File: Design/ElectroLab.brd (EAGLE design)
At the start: 175 x 100 mm, 232 parts, among them IC1 LM2902DT, IC10 CD4511BNSR, IC11 PAM8403, IC13 ADXL337, IC14 MIC5205, IC2 LM2902DT, IC3 SN74LV08ADR, IC4 SN74LV32ADR, IC5 SN74LV04ADR, IC6 4027D, IC7 4027D, IC8 NE555D, U1 USB, U2 GAS_SENSOR

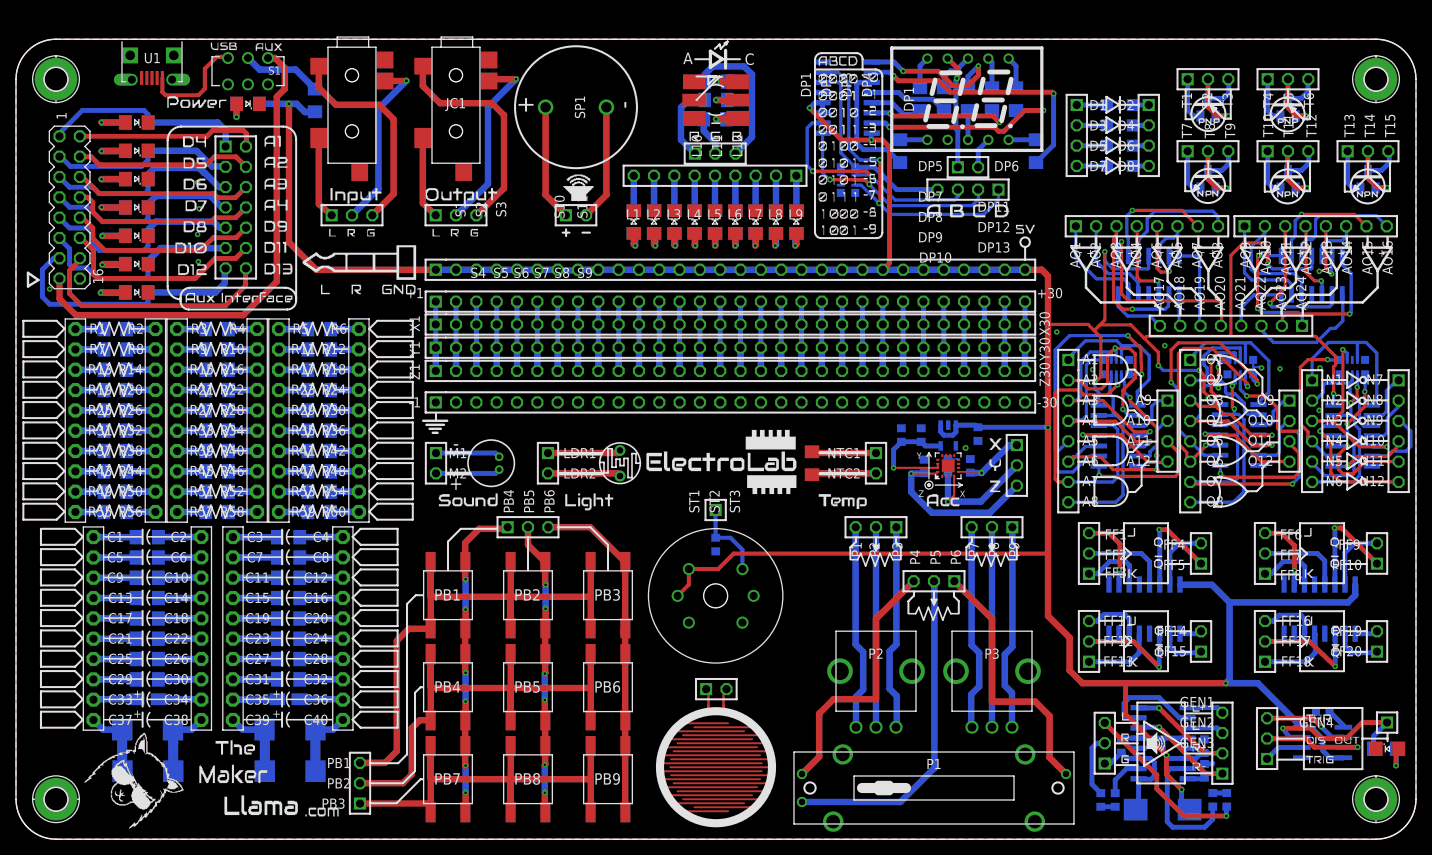
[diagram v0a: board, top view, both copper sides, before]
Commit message: Updated V3R1
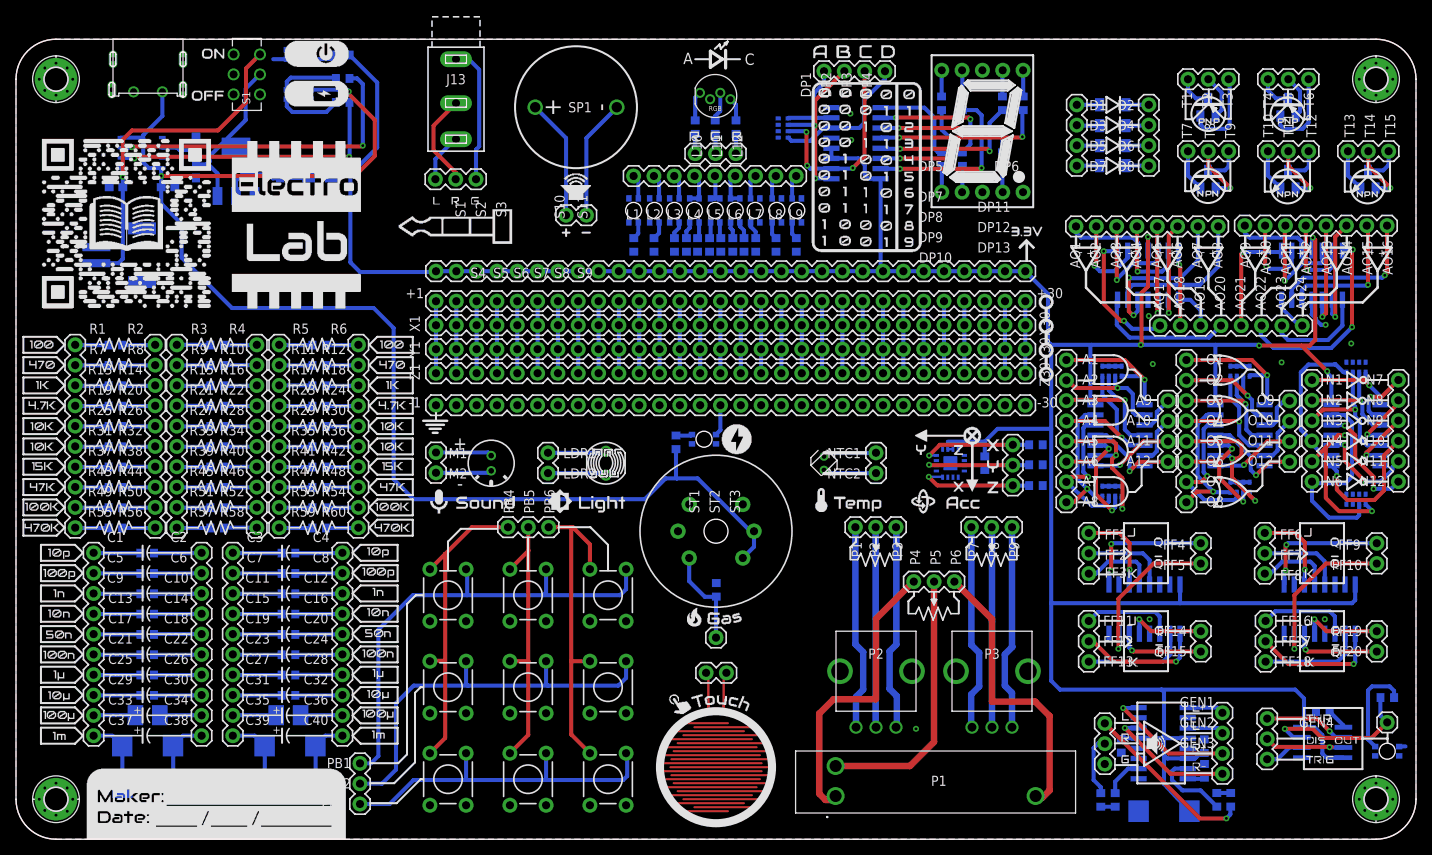
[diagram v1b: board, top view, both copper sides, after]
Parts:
- removed AR1, AR2, AR3, AR4: 1K, SpaceDIY:RESISTOR_ARRAY_X8_CAY17
- removed C33, C34: 10uF, SpaceDIY_passive_components:0603
- removed D1, D2, D3, D4: (no value), Seeed-OPL-Diode:LED-1206
- removed DP1: 2X7_SEGMENT_COMMON_CATODE_12_PINS, SpaceDIY:2X7_SEGMENT_COMMON_CATODE_12_PINS
- removed IC1, IC2: LM2902DT, Texas Instruments_By_element14_Batch_1:SOIC127P600X175-14N
- removed IC10: CD4511BNSR, SpaceDIY:SN74LS247D
- removed IC5: SN74LV04ADR, Texas Instruments_By_element14_Batch_1:SOIC127P600X175-14N
- removed JC1, JC2: SWTCHCRFT_3.5JACK5-JACK-SMD, jmsaavedra:4-JACK-SMD
- removed L0, L1, L2, L3, L4, L5, L6, L7: (no value), adafruit:1206
- removed L10, L17, L8, L9: Grn, adafruit:1206
- removed L11, L12, L13: Ylw, adafruit:1206
- removed L14, L15, L16: Red, adafruit:1206
- removed LDR: (no value), photo-elements:TO-5_V10
- removed LED_: (no value), SpaceDIY_passive_components:PLCC-6
- removed PB1, PB2, PB3, PB4, PB5, PB6, PB7, PB8, PB9: (no value), Seeed-OPL-Switch:SW4-SMD-6.0X6.0X5.0MM
- removed PH10, PH2, PH21, PH3, PH4, PH5, PH6, PH7, PH8, PH9: (no value), pinhead:1X02
- removed PH11, PH14, PH15, PH16, PH17, PH18, PH19, PH20, PH22, PH23, PH24, PH25, PH26, PH27, PH28, PH29, PH30, PH38, PH64: (no value), pinhead:1X03
- removed PH31, PH58, PH59, PH60, PH61, PH62: (no value), pinhead:1X30
- removed PH32, PH33, PH35, PH36, PH37, PH65: (no value), pinhead:1X04
- removed PH34: (no value), pinhead:1X01
- removed PH39, PH40: (no value), pinhead:1X06
- removed PH41: (no value), pinhead:2X07
- removed PH42, PH43, PH44, PH45, PH46: (no value), pinhead:1X08
- removed PH47: (no value), pinhead:1X09
- removed PH48, PH49, PH50, PH51, PH52, PH53, PH54, PH55, PH56, PH57: (no value), adafruit:1X10-BIG
- removed PH63: (no value), con-lstb:MA08-2
- added ARR1, ARR2, ARR3, ARR4, ARR5, ARR6, ARR7: 4_RES_ARRAY_R06031KOHM, SpaceDIY_passive_components:0603-ARC
- added C28, C37, C38, C39: 10uF, rcl:C0603
- added D5, D6, D7, D8: LL4148, SpaceDIY_semiconductors:LL-34
- added IC15: 74HC32S14-13, SpaceDIY_IC:SO14
- added IC9: TP4056, TP4056:SOT23-8
- added J1: (no value), SpaceDIY_connectors:JST-2-SMD
- added J10, J11, J12, J2, J4, J5, J6, J7, J8, J9: (no value), SpaceDIY_connectors:1X10
- added J13: AUDIO_JACK_MONO_3.5LCSC, SpaceDIY_connectors:PJ316
- added J14, J15, J16, J17, J18, J19: (no value), SpaceDIY_connectors:1X30
- added J20, J21, J22, J23, J24, J25, J26, J27, J28, J29, J30, J31, J32, J33, J34, J35, J36, J37: (no value), SpaceDIY_connectors:1X03
- added J3, J43, J44, J52, J53, J55: (no value), SpaceDIY_connectors:1X04
- added J38, J39, J40, J41, J47, J48, J49, J50, J54: (no value), SpaceDIY_connectors:1X02
- added J42, J51: (no value), SpaceDIY_connectors:1X01
- added J45, J46: (no value), SpaceDIY_connectors:1X06
- added J56: (no value), SpaceDIY_connectors:1X09
- added LED1, LED10, LED11, LED12, LED13, LED2, LED3, LED4, LED5, LED6, LED7, LED8, LED9: E6CC1205RYGC2UDA, SpaceDIY_semiconductors:BICOLOR_LED
- added RGB: CLEAR, SpaceDIY_semiconductors:LED-RGB-THRU
- added S10, S2, S3, S4, S5, S6, S7, S8, S9: MOMENTARY-SWITCH-SPST-PTH-6.0MM, SparkFun-Switches:TACTILE_SWITCH_PTH_6.0MM
- added U$1: FJ5101AG, SpaceDIY_semiconductors:7-SEGMENT
- added U$2, U$3, U$4, U$5, U$6: CONN_08, SpaceDIY_connectors:1X08
- added U$7: CD4511BNSR, SpaceDIY_IC:SO16
- added U3: AMS1117-3.3VSMD, SpaceDIY_IC:SOT223
- added X8: USB-C-POWER, SpaceDIY_connectors:USB-C-POWER
- C1, C10, C11, C12, C13, C14, C15, C16, C2, C3, C4, C5, C6, C7, C8, C9: device resistor:C1206 -> SpaceDIY_passive_components:0603
- C17, C18: device rcl:A/3216-18R -> SpaceDIY_passive_components:B/3528-21R
- C19, C20, C35, C36: device rcl:D/7343-31R -> SpaceDIY_passive_components:D/7343-31R
- C27: device rcl:D/7343-31W -> SpaceDIY_passive_components:D/7343-31R
- C29, C30, C31: value 10nF -> 0.1uF
- C32: value 100nF -> 0.1uF
- H1, H2, H3, H4: value (none) -> MOUNT-PAD-ROUND2.8
- IC13: value ADXL337 -> 74HC08DD; device SpaceDIY_IC:LFCSP-3X3 -> SpaceDIY_IC:SO14
- IC14: value MIC5205 -> 74HC04DD; device SparkFun:SOT23-5 -> SpaceDIY_IC:SO14
- IC3: value SN74LV08ADR -> LM324DTD; device Texas Instruments_By_element14_Batch_1:SOIC127P600X175-14N -> SpaceDIY_IC:SO14
- IC4: value SN74LV32ADR -> LM324DTD; device Texas Instruments_By_element14_Batch_1:SOIC127P600X175-14N -> SpaceDIY_IC:SO14
- IC6, IC7: value 4027D -> MC74HC112ADR2G; device 40xx:SO16 -> SpaceDIY_IC:SO16
- IC8: value NE555D -> TLC555CDR
- MIC: value ELECTRET_MICROPHON-WM-64PC/64PK -> MICROPHONE; device microphon:WM-64PC/64PK -> SpaceDIY_sensors:MICROPHONE
- NTC: device adafruit:R1206@1 -> SpaceDIY_sensors:NTC
- P1: value (none) -> SLIDE_POT_20MM; device SpaceDIY:SLIDE_POT_20MM -> SpaceDIY_electromechanical:RS201111J011
- PH1: value (none) -> PHOTORESISTOR; device pinhead:1X01 -> SpaceDIY_sensors:GL5516
- PH12: device pinhead:1X03 -> SpaceDIY_connectors:1X03
- R1, R10, R11, R12, R13, R14, R15, R16, R17, R18, R19, R2, R20, R21, R22, R23, R24, R25, R26, R27, R28, R29, R3, R30, R31, R35, R36, R37, R38, R39, R4, R41, R42, R43, R44, R45, R46, R47, R48, R49, R5, R50, R51, R52, R53, R54, R55, R56, R57, R58, R59, R6, R7, R8, R9: device resistor:R1206 -> SpaceDIY_passive_components:0603
- R32: value 330 -> 1.2k; device resistor:R1206 -> rcl:R0603
- R33: value 330 -> 1K; device resistor:R1206 -> SpaceDIY_passive_components:0603
- R34: value 330 -> 1k; device resistor:R1206 -> SpaceDIY_passive_components:0603
- SP1: value 32MM_SPEAKER -> SPEAKERFS1508MB0810-H8.0; device SpaceDIY:32MM_SPEAKER -> SpaceDIY_electromechanical:FS1508MB0810-H8.0
- T1: value (none) -> MMBT2222A; device transistor:SOT23-BEC -> SpaceDIY_semiconductors:SOT23
- T2, T3: value (none) -> T_NPNMMBT2222A-1P_CHANGJ_SOT23-BEC; device transistor:SOT23-BEC -> SpaceDIY_semiconductors:SOT23
- T4, T5: value (none) -> T_PNPMMBT5401_CHANGJ_SOT23-BEC; device transistor:SOT23-BCE -> SpaceDIY_semiconductors:SOT23
- U$16: device SpaceDIY:RESISTIVE_SENSOR_PAD -> SpaceDIY_sensors:RESISTIVE_SENSOR_PAD
- U1: value USB -> ADXL335; device daspilker:FCI-10103594-0001LF -> SparkFun-Sensors:LFCSP-16-4X4
- U2: device SparkFun:MQ-3 -> SpaceDIY_sensors:GAS_SENSOR
- moved U1 112.9 mm to (116.8, 47.0), flipped to the bottom, turned to 0 degrees
- moved PH1 102.9 mm to (73.7, 47.0), turned to 270 degrees
- moved R37 74.5 mm to (89.6, 74.3), turned to 90 degrees
- moved R36 71.6 mm to (86.7, 74.3), turned to 90 degrees
- moved R38 70.0 mm to (82.5, 49.6), turned to 270 degrees
- moved R35 68.9 mm to (83.8, 74.3), turned to 90 degrees
- moved IC14 51.0 mm to (167.5, 50.5), turned to 270 degrees
- moved R34 27.5 mm to (40.9, 92.1)
- moved R33 27.3 mm to (40.9, 95.1)
- moved IC4 26.4 mm to (162.0, 70.5), turned to 180 degrees
- moved IC3 24.7 mm to (141.5, 70.5), turned to 180 degrees
- moved IC13 21.8 mm to (138.0, 50.5), flipped to the bottom, turned to 270 degrees
- moved C31 14.2 mm to (127.5, 44.2), turned to 180 degrees
- moved R31 13.3 mm to (40.9, 98.0)
- moved R43 12.8 mm to (123.3, 85.0), turned to 270 degrees
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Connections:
- removed net 3.3V: C32.1, C33.1, IC13.14, IC13.15, IC14.5
- removed net D0: PH41.1, PH63.1, R32.2
- removed net D1: PH41.2, PH63.2
- removed net D10: PH41.11, PH63.11, R37.2
- removed net D11: PH41.12, PH63.12
- removed net D12: PH41.13, PH63.13, R38.2
- removed net D13: PH41.14, PH63.14
- removed net D2: PH41.3, PH63.3, R33.2
- removed net D3: PH41.4, PH63.4
- removed net D4: PH41.5, PH63.5, R34.2
- removed net D5: PH41.6, PH63.6
- removed net D6: PH41.7, PH63.7, R35.2
- removed net D7: PH41.8, PH63.8
- removed net D8: PH41.9, PH63.9, R36.2
- removed net D9: PH41.10, PH63.10
- removed net DG1: DP1.9, PH3.1
- removed net DG2: DP1.4, PH3.2
- removed net DP: DP1.2
- removed net JC1: JC1.2, PH12.2
- removed net JC2: JC2.2, PH64.2
- removed net N$121: JC2.3, PH64.1
- removed net N$228: PB1.1, PB1.2, PB2.1, PB2.2, PB3.1, PB3.2, PH19.3
- removed net N$229: PB4.1, PB4.2, PB5.1, PB5.2, PB6.1, PB6.2, PH19.2
- removed net N$230: PB7.1, PB7.2, PB8.1, PB8.2, PB9.1, PB9.2, PH19.1
- removed net N$233: PB3.3, PB3.4, PB6.3, PB6.4, PB9.3, PB9.4, PH20.3
- removed net N$292: L8.A, R48.1
- removed net N$300: L9.A, R49.1
- removed net N$301: L10.A, R50.1
- removed net N$302: L11.A, R51.1
- removed net N$303: L12.A, R52.1
- removed net N$304: L13.A, R53.1
- removed net N$305: L14.A, R54.1
- removed net N$306: L15.A, R55.1
- removed net N$307: L16.A, R56.1
- removed net VEXT: PH63.15, S1.1
- removed net VUSB: S1.3, U1.1
- new net N$182: LED5.1, R49.2
- new net N$185: LED6.1, R50.2
- new net N$204: LED7.1, R51.2
- new net N$214: LED8.1, R52.2
- new net N$215: LED9.1, R53.2
- new net N$216: LED7.4, R35.2
- new net N$246: LED8.4, R36.2
- new net N$247: LED9.4, R37.2
- new net N$248: LED10.4, R54.2
- new net N$251: LED11.4, R55.2
- new net N$252: LED12.4, R56.2
- new net N$253: J20.3, S2.1, S3.1, S4.1
- new net N$258: J20.2, S5.1, S6.1, S7.1
- new net N$260: J21.3, S10.3, S4.3, S7.3
- new net N$261: J20.1, S10.1, S8.1, S9.1
- new net VBAT: C28.1, IC9.5, J1.1, S1.4
- new net VIN: C37.1, IC9.4, IC9.8, LED1.2, LED1.3, R38.2, U2.A1, U2.HA, X8.VBUS
- new net VOUT: C39.1, F1.2, U3.2
- net A1A: now also ARR1.1, IC13.1, U$2.1; no longer AR1.9, IC3.1, PH45.1
- net A1B: now also ARR1.2, IC13.2, U$2.2; no longer AR1.8, IC3.2, PH45.2
- net A1Y: now also IC13.3, J52.1; no longer IC3.3, PH36.1
- net A2A: now also ARR1.3, IC13.4, U$2.3; no longer AR1.7, IC3.4, PH45.3
- net A2B: now also ARR1.4, IC13.5, U$2.4; no longer AR1.6, IC3.5, PH45.4
- net A2Y: now also IC13.6, J52.2; no longer IC3.6, PH36.2
- net A3A: now also ARR2.1, IC13.9, U$2.5; no longer AR1.1, IC3.9, PH45.5
- net A3B: now also ARR2.2, IC13.10, U$2.6; no longer AR1.2, IC3.10, PH45.6
- net A3Y: now also IC13.8, J52.3; no longer IC3.8, PH36.3
- net A4A: now also ARR2.3, IC13.12, U$2.7; no longer AR1.3, IC3.12, PH45.7
- net A4B: now also ARR2.4, IC13.13, U$2.8; no longer AR1.4, IC3.13, PH45.8
- net A4Y: now also IC13.11, J52.4; no longer IC3.11, PH36.4
- net B: now also J37.3; no longer PH11.3
- net G: now also J37.2, R58.2; no longer PH11.2, R57.2
- net GND: now also ARR1.5, ARR1.6, ARR1.7, ARR1.8, ARR2.5, ARR2.6, ARR2.7, ARR2.8, ARR3.5, ARR3.6, ARR3.7, ARR3.8, ARR4.5, ARR4.6, ARR4.7, ARR4.8, ARR5.5, ARR5.6, ARR5.7, ARR5.8, ARR6.7, ARR6.8, ARR7.5, ARR7.6, ARR7.7, ARR7.8, C28.2, C37.2, C38.2, C39.2, IC14.7, IC15.7, IC3.11, IC4.11, IC6.10, IC6.14, IC6.15, IC7.10, IC7.14, IC7.15, IC9.1, IC9.3, J1.2, J14.1, J14.10, J14.11, J14.12, J14.13, J14.14, J14.15, J14.16, J14.17, J14.18, J14.19, J14.2, J14.20, J14.21, J14.22, J14.23, J14.24, J14.25, J14.26, J14.27, J14.28, J14.29, J14.3, J14.30, J14.4, J14.5, J14.6, J14.7, J14.8, J14.9, J36.1, LED13.1, LED2.1, LED3.1, R32.1, R35.1, R36.1, R37.1, R48.1, R49.1, R50.1, R51.1, R52.1, R53.1, R54.1, R55.1, R56.1, RGB.C, U$1.3, U$1.8, U$7.5, U$7.8, U1.3, U1.6, U1.7, U3.1, X8.GND; no longer AR1.10, AR1.5, AR2.10, AR2.5, AR3.10, AR3.5, AR4.10, AR4.5, C33.2, C34.2, IC1.11, IC10.GND, IC10.RBI, IC13.6, IC14.2, IC2.11, IC3.7, IC4.7, IC5.7, IC6.12, IC6.7, IC6.9, IC7.12, IC7.7, IC7.9, L0.C, L1.C, L10.C, L11.C, L12.C, L13.C, L14.C, L15.C, L16.C, L17.C, L2.C, L3.C, L4.C, L5.C, L6.C, L7.C, L8.C, L9.C, LED_.4, LED_.5, LED_.6, PH38.1, PH62.1, PH62.10, PH62.11, PH62.12, PH62.13, PH62.14, PH62.15, PH62.16, PH62.17, PH62.18, PH62.19, PH62.2, PH62.20, PH62.21, PH62.22, PH62.23, PH62.24, PH62.25, PH62.26, PH62.27, PH62.28, PH62.29, PH62.3, PH62.30, PH62.4, PH62.5, PH62.6, PH62.7, PH62.8, PH62.9, PH63.16
- net I1A: now also ARR5.1, IC14.1, J45.1; no longer AR3.9, IC5.1, PH39.1
- net I1Y: now also IC14.2, J46.1; no longer IC5.2, PH40.1
- net I2A: now also ARR5.2, IC14.3, J45.2; no longer AR3.3, IC5.3, PH39.2
- net I2Y: now also IC14.4, J46.2; no longer IC5.4, PH40.2
- net I3A: now also ARR5.3, IC14.5, J45.3; no longer AR3.7, IC5.5, PH39.3
- net I3Y: now also IC14.6, J46.3; no longer IC5.6, PH40.3
- net I4A: now also ARR5.4, IC14.9, J45.4; no longer AR3.6, IC5.9, PH39.4
- net I4Y: now also IC14.8, J46.4; no longer IC5.8, PH40.4
- net I5A: now also ARR6.1, IC14.11, J45.5; no longer AR3.1, IC5.11, PH39.5
- net I5Y: now also IC14.10, J46.5; no longer IC5.10, PH40.5
- net I6A: now also ARR6.2, IC14.13, J45.6; no longer AR3.2, IC5.13, PH39.6
- net I6Y: now also IC14.12, J46.6; no longer IC5.12, PH40.6
- net IA: now also ARR7.1, J55.1, U$7.7; no longer AR4.9, IC10.IA, PH35.1
- net IB: now also ARR7.2, J55.2, U$7.1; no longer AR4.8, IC10.IB, PH35.2
- net IC: now also ARR7.3, J55.3, U$7.2; no longer AR4.7, IC10.IC, PH35.3
- net ID: now also ARR7.4, J55.4, U$7.6; no longer AR4.6, IC10.ID, PH35.4
- net IN_L: now also J36.3; no longer PH38.3
- net IN_R: now also J36.2; no longer PH38.2
- net L1: now also J56.1, LED4.2; no longer PH47.9, R48.2
- net L2: now also J56.2, LED5.2; no longer PH47.8, R49.2
- net L3: now also J56.3, LED6.2; no longer PH47.7, R50.2
- net L4: now also J56.4, LED7.2, LED7.3; no longer PH47.6, R51.2
- net L5: now also J56.5, LED8.2, LED8.3; no longer PH47.5, R52.2
- net L6: now also J56.6, LED9.2, LED9.3; no longer PH47.4, R53.2
- net L7: now also J56.7, LED10.3; no longer PH47.3, R54.2
- net L8: now also J56.8, LED11.3; no longer PH47.2, R55.2
- net L9: now also J56.9, LED12.3; no longer PH47.1, R56.2
- net N$1: now also J2.1; no longer PH48.10
- net N$10: now also J2.10; no longer PH48.1
- net N$100: now also J12.1; no longer PH55.1
- net N$101: now also D8.A, J53.4; no longer D4.+, PH32.4
- net N$102: now also J13.2, PH12.2; no longer L1.A, R32.1
- net N$103: now also LED2.2; no longer L0.A
- net N$104: now also IC9.6, R34.2; no longer L2.A, R33.1
- net N$105: now also LED1.4, R33.1; no longer L3.A, R34.1
- net N$106: now also LED1.1, R34.1; no longer L4.A, R35.1
- net N$107: now also IC9.2, R32.2; no longer L5.A, R36.1
- net N$108: now also IC9.7, R33.2; no longer L6.A, R37.1
- net N$109: now also C38.1, S1.5, U3.3; no longer L7.A, R38.1
- net N$11: now also J4.10; no longer PH49.10
- net N$110: now also D8.C, J44.4; no longer D4.-, PH33.4
- net N$111: now also D5.A, J53.1; no longer D1.+, PH32.1
- net N$112: now also IC6.5, J47.1; no longer IC6.1, PH9.2
- net N$113: now also IC6.9, J48.1; no longer IC6.15, PH7.2
- net N$114: now also IC7.5, J49.1; no longer IC7.1, PH10.2
- net N$115: now also IC7.9, J50.1; no longer IC7.15, PH8.2
- net N$116: now also J13.1; no longer JC1.3
- net N$117: now also RGB.G; no longer LED_.2
- net N$118: now also LED4.1, R48.2; no longer F1.1, S1.2
- net N$119: now also J42.1; no longer PH34.1
- net N$12: now also J4.9; no longer PH49.9
- net N$120: now also LED13.2, R38.1; no longer JC2.1, PH64.3
- net N$122: now also LED3.2; no longer L17.A
- net N$125: now also J41.2; no longer PH21.1
- net N$126: now also J41.1; no longer PH21.2
- net N$127: now also J15.24, J16.24, J17.24, J18.24; no longer PH31.7, PH59.7, PH60.7, PH61.7
- net N$128: now also J15.30, J16.30, J17.30, J18.30; no longer PH31.1, PH59.1, PH60.1, PH61.1
- net N$129: now also J15.29, J16.29, J17.29, J18.29; no longer PH31.2, PH59.2, PH60.2, PH61.2
- net N$13: now also J4.8; no longer PH49.8
- net N$130: now also IC3.3, U$4.1; no longer IC1.13, PH42.1
- net N$131: now also IC3.2, U$4.2; no longer IC1.12, PH42.2
- net N$132: now also IC3.5, U$4.3; no longer IC1.9, PH42.3
- net N$133: now also IC3.6, U$4.4; no longer IC1.10, PH42.4
- net N$134: now also IC3.10, U$4.5; no longer IC1.6, PH42.5
- net N$135: now also IC3.9, U$4.6; no longer IC1.5, PH42.6
- net N$136: now also IC3.12, U$4.7; no longer IC1.2, PH42.7
- net N$137: now also IC3.13, U$4.8; no longer IC1.3, PH42.8
- net N$138: now also IC4.3, U$5.1; no longer IC2.13, PH43.1
- net N$139: now also J15.28, J16.28, J17.28, J18.28; no longer PH31.3, PH59.3, PH60.3, PH61.3
- net N$14: now also J4.7; no longer PH49.7
- net N$140: now also J15.27, J16.27, J17.27, J18.27; no longer PH31.4, PH59.4, PH60.4, PH61.4
- net N$141: now also J15.26, J16.26, J17.26, J18.26; no longer PH31.5, PH59.5, PH60.5, PH61.5
- net N$142: now also J15.25, J16.25, J17.25, J18.25; no longer PH31.6, PH59.6, PH60.6, PH61.6
- net N$143: now also J15.23, J16.23, J17.23, J18.23; no longer PH31.8, PH59.8, PH60.8, PH61.8
- net N$144: now also J15.22, J16.22, J17.22, J18.22; no longer PH31.9, PH59.9, PH60.9, PH61.9
- net N$145: now also J15.21, J16.21, J17.21, J18.21; no longer PH31.10, PH59.10, PH60.10, PH61.10
- net N$146: now also IC6.2, J26.1; no longer IC6.5, PH27.1
- net N$147: now also J15.20, J16.20, J17.20, J18.20; no longer PH31.11, PH59.11, PH60.11, PH61.11
- net N$148: now also J15.19, J16.19, J17.19, J18.19; no longer PH31.12, PH59.12, PH60.12, PH61.12
- net N$149: now also J15.18, J16.18, J17.18, J18.18; no longer PH31.13, PH59.13, PH60.13, PH61.13
- net N$15: now also J4.5; no longer PH49.5
- net N$150: now also J15.17, J16.17, J17.17, J18.17; no longer PH31.14, PH59.14, PH60.14, PH61.14
- net N$151: now also J15.16, J16.16, J17.16, J18.16; no longer PH31.15, PH59.15, PH60.15, PH61.15
- net N$152: now also J15.15, J16.15, J17.15, J18.15; no longer PH31.16, PH59.16, PH60.16, PH61.16
- net N$153: now also J15.14, J16.14, J17.14, J18.14; no longer PH31.17, PH59.17, PH60.17, PH61.17
- net N$154: now also J15.13, J16.13, J17.13, J18.13; no longer PH31.18, PH59.18, PH60.18, PH61.18
- net N$155: now also IC6.1, J26.2; no longer IC6.3, PH27.2
- net N$156: now also IC6.3, J26.3; no longer IC6.6, PH27.3
- net N$157: now also IC6.12, J27.1; no longer IC6.11, PH25.1
- net N$158: now also J27.2; no longer PH25.2
- net N$159: now also IC6.11, J27.3; no longer IC6.10, PH25.3
- net N$16: now also J4.6; no longer PH49.6
- net N$160: now also IC7.2, J28.1; no longer IC7.5, PH28.1
- net N$161: now also IC7.1, J28.2; no longer IC7.3, PH28.2
- net N$162: now also IC7.3, J28.3; no longer IC7.6, PH28.3
- net N$163: now also J15.12, J16.12, J17.12, J18.12; no longer PH31.19, PH59.19, PH60.19, PH61.19
- net N$164: now also J15.11, J16.11, J17.11, J18.11; no longer PH31.20, PH59.20, PH60.20, PH61.20
- net N$165: now also J15.10, J16.10, J17.10, J18.10; no longer PH31.21, PH59.21, PH60.21, PH61.21
- net N$166: now also J15.9, J16.9, J17.9, J18.9; no longer PH31.22, PH59.22, PH60.22, PH61.22
- net N$167: now also J15.8, J16.8, J17.8, J18.8; no longer PH31.23, PH59.23, PH60.23, PH61.23
- net N$168: now also J15.7, J16.7, J17.7, J18.7; no longer PH31.24, PH59.24, PH60.24, PH61.24
- net N$169: now also J15.6, J16.6, J17.6, J18.6; no longer PH31.25, PH59.25, PH60.25, PH61.25
- net N$17: now also J4.4; no longer PH49.4
- net N$170: now also J15.5, J16.5, J17.5, J18.5; no longer PH31.26, PH59.26, PH60.26, PH61.26
- net N$171: now also IC7.12, J29.1; no longer IC7.11, PH26.1
- net N$172: now also J29.2; no longer PH26.2
- net N$173: now also IC7.11, J29.3; no longer IC7.10, PH26.3
- net N$174: now also J15.4, J16.4, J17.4, J18.4; no longer PH31.27, PH59.27, PH60.27, PH61.27
- net N$175: now also J15.3, J16.3, J17.3, J18.3; no longer PH31.28, PH59.28, PH60.28, PH61.28
- net N$176: now also J15.2, J16.2, J17.2, J18.2; no longer PH31.29, PH59.29, PH60.29, PH61.29
- net N$177: now also J15.1, J16.1, J17.1, J18.1; no longer PH31.30, PH59.30, PH60.30, PH61.30
- net N$178: now also IC6.6, J47.2; no longer IC6.2, PH9.1
- net N$179: now also IC6.7, J48.2; no longer IC6.14, PH7.1
- net N$18: now also J4.3; no longer PH49.3
- net N$180: now also IC7.6, J49.2; no longer IC7.2, PH10.1
- net N$181: now also IC7.7, J50.2; no longer IC7.14, PH8.1
- net N$183: now also D7.A, J53.3; no longer D3.+, PH32.3
- net N$184: now also D6.A, J53.2; no longer D2.+, PH32.2
- net N$186: now also IC4.2, U$5.2; no longer IC2.12, PH43.2
- net N$187: now also IC4.5, U$5.3; no longer IC2.9, PH43.3
- net N$188: now also IC4.6, U$5.4; no longer IC2.10, PH43.4
- net N$189: now also IC4.10, U$5.5; no longer IC2.6, PH43.5
- net N$19: now also J4.2; no longer PH49.2
- net N$190: now also IC4.9, U$5.6; no longer IC2.5, PH43.6
- net N$191: now also IC4.12, U$5.7; no longer IC2.2, PH43.7
- net N$192: now also IC4.13, U$5.8; no longer IC2.3, PH43.8
- net N$193: now also IC3.1, U$6.1; no longer IC1.14, PH44.8
- net N$194: now also IC3.7, U$6.2; no longer IC1.8, PH44.7
- net N$195: now also IC3.8, U$6.3; no longer IC1.7, PH44.6
- net N$196: now also IC3.14, U$6.4; no longer IC1.1, PH44.5
- net N$197: now also IC4.1, U$6.5; no longer IC2.14, PH44.4
- net N$198: now also IC4.7, U$6.6; no longer IC2.8, PH44.3
- net N$199: now also D5.C, J44.1; no longer D1.-, PH33.1
- net N$2: now also J2.2; no longer PH48.9
- net N$20: now also J4.1; no longer PH49.1
- net N$200: now also IC4.8, U$6.7; no longer IC2.7, PH44.2
- net N$201: now also IC4.14, U$6.8; no longer IC2.1, PH44.1
- net N$202: now also D6.C, J44.2; no longer D2.-, PH33.2
- net N$203: now also D7.C, J44.3; no longer D3.-, PH33.3
- net N$205: now also J31.1, T1.2; no longer PH16.1, T1.E
- net N$206: now also J31.2, T1.1; no longer PH16.2, T1.B
- net N$207: now also J31.3, T1.3; no longer PH16.3, T1.C
- net N$208: now also J32.1, T2.2; no longer PH17.1, T2.E
- net N$209: now also J32.2, T2.1; no longer PH17.2, T2.B
- net N$21: now also J5.1; no longer PH50.10
- net N$210: now also J32.3, T2.3; no longer PH17.3, T2.C
- net N$211: now also J33.1, T3.2; no longer PH18.1, T3.E
- net N$212: now also J33.2, T3.1; no longer PH18.2, T3.B
- net N$213: now also J33.3, T3.3; no longer PH18.3, T3.C
- net N$217: now also J34.1, T4.3; no longer PH14.1, T4.C
- net N$218: now also J34.2, T4.1; no longer PH14.2, T4.B
- net N$219: now also J34.3, T4.2; no longer PH14.3, T4.E
- net N$22: now also J5.2; no longer PH50.9
- net N$220: now also J35.1, T5.3; no longer PH15.1, T5.C
- net N$221: now also J35.2, T5.1; no longer PH15.2, T5.B
- net N$222: now also J35.3, T5.2; no longer PH15.3, T5.E
- net N$223: now also J30.1; no longer PH29.1
- net N$224: now also J51.1; no longer PH1.1
- net N$226: now also J30.2; no longer PH29.2
- net N$227: now also J30.3; no longer PH29.3
- net N$23: now also J5.3; no longer PH50.8
- net N$231: now also J21.1, S2.3, S5.3, S8.3; no longer PB1.3, PB1.4, PB4.3, PB4.4, PB7.3, PB7.4, PH20.1
- net N$232: now also J21.2, S3.3, S6.3, S9.3; no longer PB2.3, PB2.4, PB5.3, PB5.4, PB8.3, PB8.4, PH20.2
- net N$234: now also J39.1, PH1.1; no longer LDR.1, PH5.1
- net N$235: now also J39.2, PH1.3; no longer LDR.2, PH5.2
- net N$236: now also J40.1; no longer PH6.1
- net N$237: now also J23.1; no longer PH22.1
- net N$238: now also J23.2; no longer PH22.2
- net N$239: now also J23.3; no longer PH22.3
- net N$24: now also J5.4; no longer PH50.7
- net N$240: now also J22.1; no longer PH24.1
- net N$241: now also J22.2; no longer PH24.2
- net N$242: now also J22.3; no longer PH24.3
- net N$243: now also J24.1; no longer PH23.1
- net N$244: now also J24.2; no longer PH23.2
- net N$245: now also J24.3; no longer PH23.3
- net N$249: now also J38.1; no longer PH4.1
- net N$25: now also J5.5; no longer PH50.6
- net N$250: now also J38.2; no longer PH4.2
- net N$256: now also J40.2; no longer PH6.2
- net N$257: now also J54.2; no longer PH2.1
- net N$26: now also J5.6; no longer PH50.5
- net N$264: now also J13.3; no longer JC1.1
- net N$27: now also J5.7; no longer PH50.4
- net N$28: now also J5.8; no longer PH50.3
- net N$29: now also J5.9; no longer PH50.2
- net N$291: now also J54.1; no longer PH2.2
- net N$3: now also J2.3; no longer PH48.8
- net N$30: now also J5.10; no longer PH50.1
- net N$308: now also RGB.R; no longer LED_.1
- net N$31: now also J6.10; no longer PH51.10
- net N$310: now also RGB.B; no longer LED_.3
- net N$32: now also J6.9; no longer PH51.9
- net N$33: now also J6.8; no longer PH51.8
- net N$34: now also J6.7; no longer PH51.7
- net N$35: now also J6.6; no longer PH51.6
- net N$36: now also J6.5; no longer PH51.5
- net N$37: now also J6.4; no longer PH51.4
- net N$38: now also J6.3; no longer PH51.3
- net N$39: now also J6.2; no longer PH51.2
- net N$4: now also J2.4; no longer PH48.7
- net N$40: now also J6.1; no longer PH51.1
- net N$41: now also J7.1; no longer PH52.10
- net N$42: now also J7.2; no longer PH52.9
- net N$43: now also J7.3; no longer PH52.8
- net N$44: now also J7.4; no longer PH52.7
- net N$45: now also J7.5; no longer PH52.6
- net N$46: now also J7.6; no longer PH52.5
- net N$47: now also J7.7; no longer PH52.4
- net N$48: now also J7.8; no longer PH52.3
- net N$49: now also J7.9; no longer PH52.2
- net N$5: now also J2.5; no longer PH48.6
- net N$50: now also J7.10; no longer PH52.1
- net N$51: now also J8.10; no longer PH53.10
- net N$52: now also J8.9; no longer PH53.9
- net N$53: now also J8.8; no longer PH53.8
- net N$54: now also J8.7; no longer PH53.7
- net N$55: now also J8.6; no longer PH53.6
- net N$56: now also J8.5; no longer PH53.5
- net N$57: now also J8.4; no longer PH53.4
- net N$58: now also J8.3; no longer PH53.3
- net N$59: now also J8.2; no longer PH53.2
- net N$6: now also J2.6; no longer PH48.5
- net N$60: now also J8.1; no longer PH53.1
- net N$61: now also J9.1; no longer PH56.10
- net N$62: now also J9.2; no longer PH56.9
- net N$63: now also J9.3; no longer PH56.8
- net N$64: now also J9.4; no longer PH56.7
- net N$65: now also J9.5; no longer PH56.6
- net N$66: now also J9.6; no longer PH56.5
- net N$67: now also J9.7; no longer PH56.4
- net N$68: now also J9.8; no longer PH56.3
- net N$69: now also J9.9; no longer PH56.2
- net N$7: now also J2.7; no longer PH48.4
- net N$70: now also J9.10; no longer PH56.1
- net N$71: now also J10.1; no longer PH57.1
- net N$72: now also J10.2; no longer PH57.2
- net N$73: now also J10.3; no longer PH57.3
- net N$74: now also J10.4; no longer PH57.4
- net N$75: now also J10.5; no longer PH57.5
- net N$76: now also J10.6; no longer PH57.6
- net N$77: now also J10.7; no longer PH57.7
- net N$78: now also J10.8; no longer PH57.8
- net N$79: now also J10.9; no longer PH57.9
- net N$8: now also J2.8; no longer PH48.3
- net N$80: now also J10.10; no longer PH57.10
- net N$81: now also J11.1; no longer PH54.10
- net N$82: now also J11.2; no longer PH54.9
- net N$83: now also J11.3; no longer PH54.8
- net N$84: now also J11.4; no longer PH54.7
- net N$85: now also J11.5; no longer PH54.6
- net N$86: now also J11.6; no longer PH54.5
- net N$87: now also J11.7; no longer PH54.4
- net N$88: now also J11.8; no longer PH54.3
- net N$89: now also J11.9; no longer PH54.2
- net N$9: now also J2.9; no longer PH48.2
- net N$90: now also J11.10; no longer PH54.1
- net N$91: now also J12.10; no longer PH55.10
- net N$92: now also J12.9; no longer PH55.9
- net N$93: now also J12.8; no longer PH55.8
- net N$94: now also J12.7; no longer PH55.7
- net N$95: now also J12.6; no longer PH55.6
- net N$96: now also J12.5; no longer PH55.5
- net N$97: now also J12.4; no longer PH55.4
- net N$98: now also J12.3; no longer PH55.3
- net N$99: now also J12.2; no longer PH55.2
- net O1A: now also ARR3.1, IC15.1, U$3.1; no longer AR2.9, IC4.1, PH46.1
- net O1B: now also ARR3.2, IC15.2, U$3.2; no longer AR2.8, IC4.2, PH46.2
- net O1Y: now also IC15.3, J43.1; no longer IC4.3, PH37.1
- net O2A: now also ARR3.3, IC15.4, U$3.3; no longer AR2.7, IC4.4, PH46.3
- net O2B: now also ARR3.4, IC15.5, U$3.4; no longer AR2.6, IC4.5, PH46.4
- net O2Y: now also IC15.6, J43.2; no longer IC4.6, PH37.2
- net O3A: now also ARR4.1, IC15.9, U$3.5; no longer AR2.1, IC4.9, PH46.5
- net O3B: now also ARR4.2, IC15.10, U$3.6; no longer AR2.2, IC4.10, PH46.6
- net O3Y: now also IC15.8, J43.3; no longer IC4.8, PH37.3
- net O4A: now also ARR4.3, IC15.12, U$3.7; no longer AR2.3, IC4.12, PH46.7
- net O4B: now also ARR4.4, IC15.13, U$3.8; no longer AR2.4, IC4.13, PH46.8
- net O4Y: now also IC15.11, J43.4; no longer IC4.11, PH37.4
- net OUT_L+: now also J3.1; no longer PH65.4
- net OUT_L-: now also J3.2; no longer PH65.3
- net OUT_R+: now also J3.3; no longer PH65.2
- net OUT_R-: now also J3.4; no longer PH65.1
- net R: now also J37.1, R57.2; no longer PH11.1, R58.2
- net SA: now also U$1.7; no longer DP1.10
- net SA': now also U$7.13; no longer IC10.A
- net SB: now also U$1.6; no longer DP1.8
- net SB': now also U$7.12; no longer IC10.B
- net SC: now also U$1.4; no longer DP1.1
- net SC': now also U$7.11; no longer IC10.C
- net SD: now also U$1.2; no longer DP1.5
- net SD': now also U$7.10; no longer IC10.D
- net SE: now also U$1.1; no longer DP1.3
- net SE': now also U$7.9; no longer IC10.E
- net SF: now also U$1.9; no longer DP1.6
- net SF': now also U$7.15; no longer IC10.F
- net SG: now also U$1.10; no longer DP1.7
- net SG': now also U$7.14; no longer IC10.G
- net VCC: now also C32.1, F1.1, IC13.14, IC14.14, IC15.14, IC3.4, IC4.4, J19.1, J19.10, J19.11, J19.12, J19.13, J19.14, J19.15, J19.16, J19.17, J19.18, J19.19, J19.2, J19.20, J19.21, J19.22, J19.23, J19.24, J19.25, J19.26, J19.27, J19.28, J19.29, J19.3, J19.30, J19.4, J19.5, J19.6, J19.7, J19.8, J19.9, U$7.16, U$7.3, U$7.4, U1.14, U1.15; no longer C34.1, F1.2, IC1.4, IC10.BI/RBO, IC10.LT, IC10.VCC, IC14.1, IC14.3, IC2.4, IC3.14, IC4.14, IC5.14, PH58.1, PH58.10, PH58.11, PH58.12, PH58.13, PH58.14, PH58.15, PH58.16, PH58.17, PH58.18, PH58.19, PH58.2, PH58.20, PH58.21, PH58.22, PH58.23, PH58.24, PH58.25, PH58.26, PH58.27, PH58.28, PH58.29, PH58.3, PH58.30, PH58.4, PH58.5, PH58.6, PH58.7, PH58.8, PH58.9, U2.A1, U2.HA
- net X+: now also J25.1, U1.12; no longer IC13.5, PH30.1
- net Y+: now also J25.2, U1.10; no longer IC13.4, PH30.2
- net Z+: now also J25.3, U1.8; no longer IC13.16, PH30.3
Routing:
- net VIN: track 0.00 -> 177.3 mm, vias 0 -> 2
- net VCC: track 491.8 -> 412.6 mm, vias 14 -> 5
- net N$228: track 77.1 -> 0.00 mm
- net N$229: track 68.5 -> 0.00 mm
- net N$230: track 63.1 -> 0.00 mm
- net VEXT: track 62.0 -> 0.00 mm
- net N$253: track 0.00 -> 60.7 mm
- net N$258: track 0.00 -> 52.0 mm
- net N$261: track 0.00 -> 44.5 mm
- net VBAT: track 0.00 -> 43.7 mm, vias 0 -> 1
- net N$233: track 42.8 -> 0.00 mm
- net N$260: track 0.00 -> 40.7 mm
- net N$108: track 5.81 -> 40.0 mm, vias 1 -> 2
- net D12: track 33.0 -> 0.00 mm
- net IA: track 43.4 -> 11.8 mm, vias 2 -> 0
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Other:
- board text added: "JLCJLCJLCJLC"
